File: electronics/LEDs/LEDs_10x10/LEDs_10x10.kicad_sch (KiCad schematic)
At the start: 105 parts, among them Q2 NPN, U1 OPA735

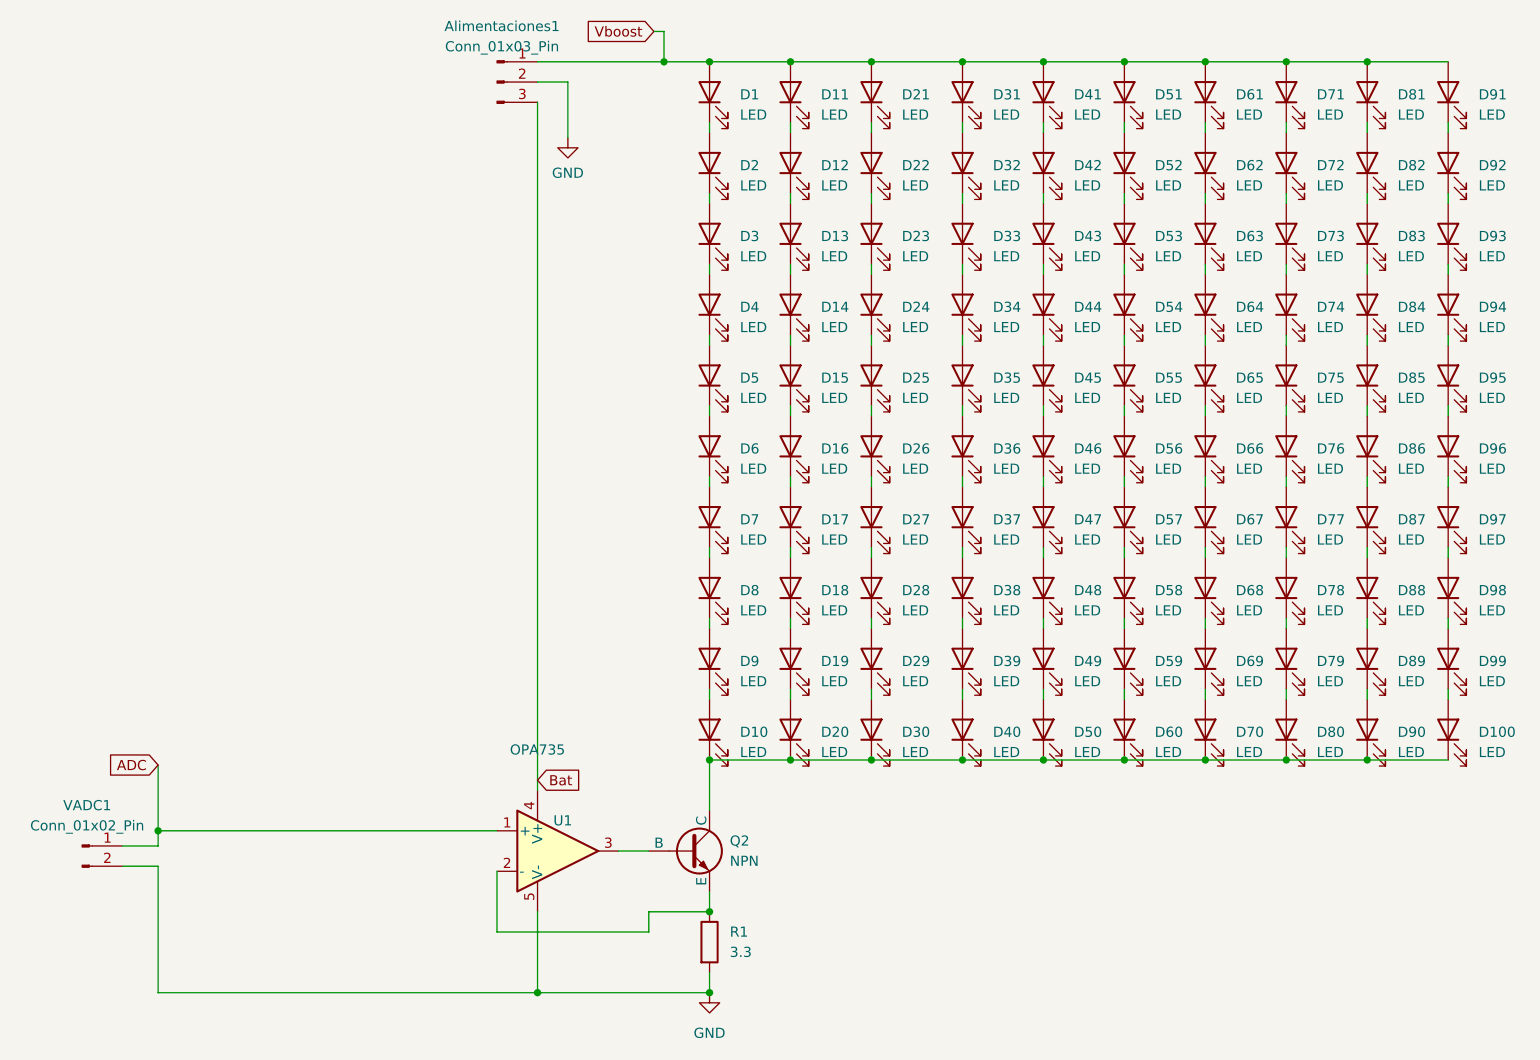
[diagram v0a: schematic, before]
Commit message: Esquematico_LEDS_Test
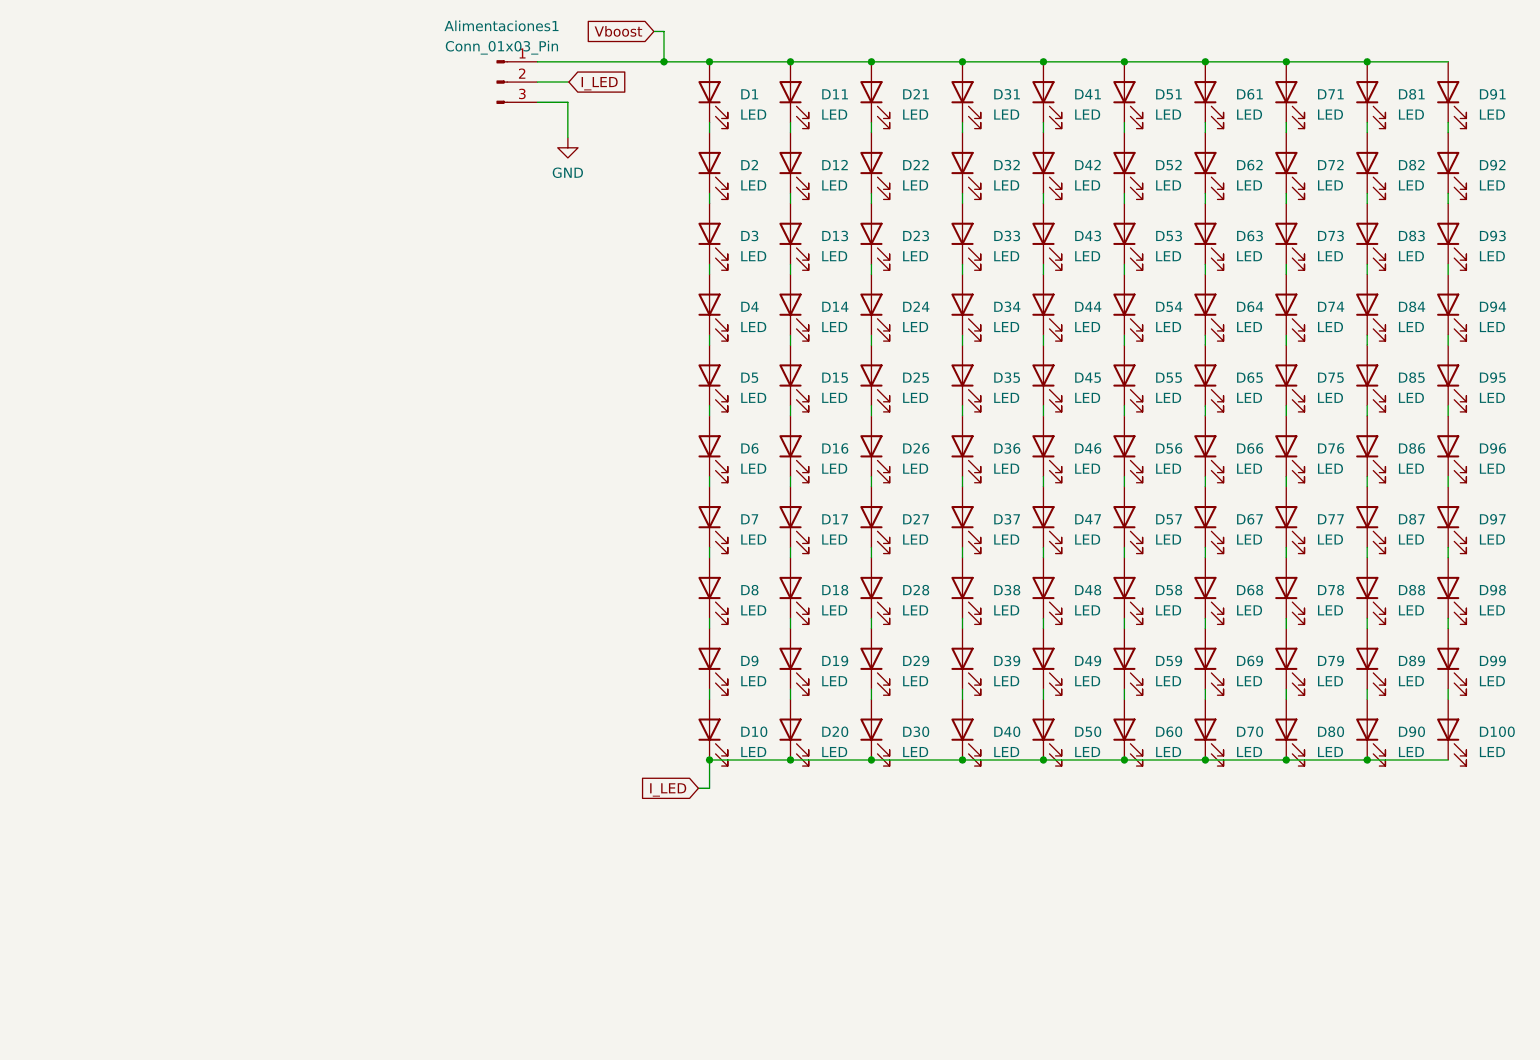
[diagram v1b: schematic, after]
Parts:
- removed Q2: NPN, Package_TO_SOT_SMD:SOT-223, symbol Simulation_SPICE:NPN
- removed R1: 3.3, Resistor_SMD:R_0603_1608Metric, symbol Device:R
- removed U1: OPA735, Package_TO_SOT_SMD:TSOT-23-5_HandSoldering, symbol Simulation_SPICE:OPAMP
- removed VADC1: Conn_01x02_Pin, Connector_JST:JST_XH_B2B-XH-A_1x02_P2.50mm_Vertical, symbol Connector:Conn_01x02_Pin
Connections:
- net Bat is gone; now on net GND: Alimentaciones1.3 (Pin_3)
- net GND: no longer Alimentaciones1.2 (Pin_2)
- net I_LED: now reaches D10.1 (K), D100.1 (K), D20.1 (K), D30.1 (K), D40.1 (K), D50.1 (K), D60.1 (K), D70.1 (K), D80.1 (K), D90.1 (K)
- net I_LED: now also Alimentaciones1.2 (Pin_2)
